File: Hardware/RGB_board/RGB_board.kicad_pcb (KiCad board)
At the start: 2 copper layers, 65 x 56.5 mm, 35 parts, among them J1 PI_HAT_3, J10 Conn_01x02, J2 Screw_Terminal_01x02, J3 Screw_Terminal_01x04, J4 Screw_Terminal_01x02, J5 Conn_01x02, J6 Conn_01x02, J7 Conn_01x02, J8 Conn_01x04, J9 Conn_01x04, Q1 Si1308EDL, Q2 Si1308EDL, Q3 Si1308EDL, Q4 Si1308EDL, SW1 SW_SPDT, SW2 SW_Push_SPST, U1 VO615A-2X009T, U2 VO615A-2X009T, U3 VO615A-2X009T

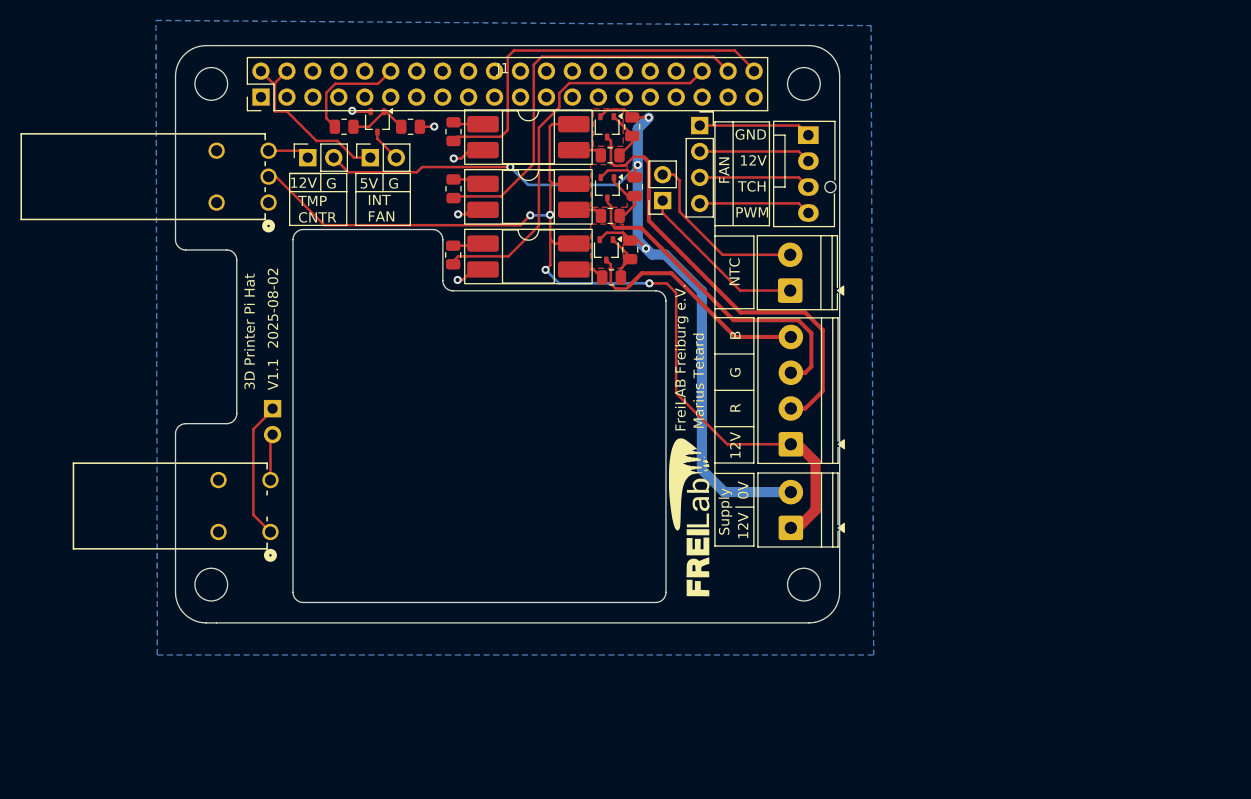
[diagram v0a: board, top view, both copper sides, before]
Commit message: große fortschritte, mockup bereit
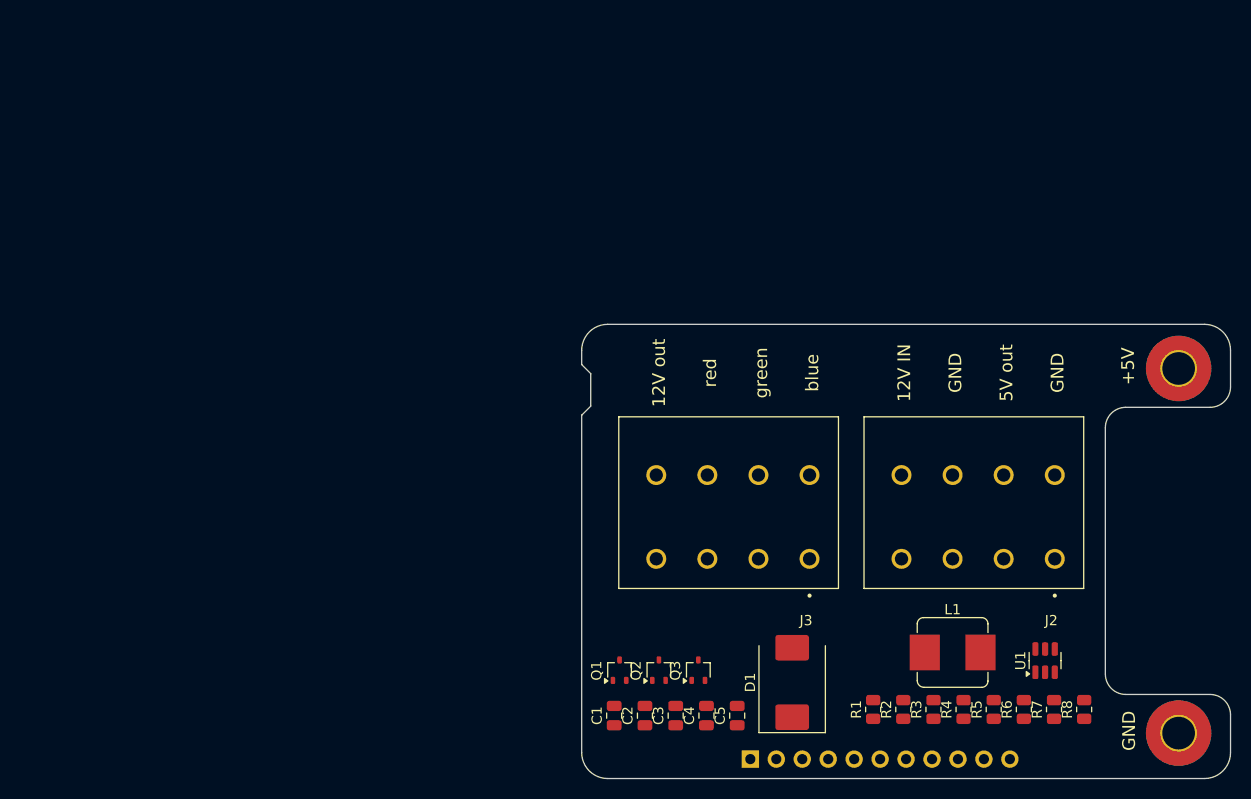
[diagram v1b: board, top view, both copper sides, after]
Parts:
- removed G***: LOGO, aa_MyParts:Freilab_Logo_4mm
- removed H3, H4: MountingHole, MountingHole:MountingHole_3.2mm_M3_DIN965
- removed J10, J5, J6, J7: Conn_01x02, Connector_PinSocket_2.54mm:PinSocket_1x02_P2.54mm_Vertical
- removed J4: Screw_Terminal_01x02, TerminalBlock_Phoenix:TerminalBlock_Phoenix_PT-1,5-2-3.5-H_1x02_P3.50mm_Horizontal
- removed J8: Conn_01x04, Connector_PinSocket_2.54mm:PinSocket_1x04_P2.54mm_Vertical
- removed J9: Conn_01x04, Connector:FanPinHeader_1x04_P2.54mm_Vertical
- removed Q4: Si1308EDL, Package_TO_SOT_SMD:SOT-323_SC-70
- removed R10, R11, R9: 1k5, Resistor_SMD:R_0805_2012Metric
- removed SW1: SW_SPDT, aa_MyParts:SW_200MSP1T1B2M6QE_EWI
- removed SW2: SW_Push_SPST, aa_MyParts:SW_800AWSP9M6QE
- removed U2, U3: VO615A-2X009T, Package_DIP:DIP-4_W8.89mm_SMDSocket_LongPads
- added C1: 10uF, Capacitor_SMD:C_0805_2012Metric, F.Cu at (119.9, 121.1)
- added C2: 10uF, Capacitor_SMD:C_0805_2012Metric, F.Cu at (122.9, 121.1)
- added C3: 100nF, Capacitor_SMD:C_0805_2012Metric, F.Cu at (126.0, 121.1)
- added C4: 22uF, Capacitor_SMD:C_0805_2012Metric, F.Cu at (129.0, 121.1)
- added C5: 22uF, Capacitor_SMD:C_0805_2012Metric, F.Cu at (132.0, 121.1)
- added D1: CDBC540-G, Diode_SMD:D_SMC, F.Cu at (137.4, 117.8)
- added L1: 3.3uH, 6A, Inductor_SMD:L_Bourns_SRP7028A_7.3x6.6mm, F.Cu at (153.1, 114.9)
- added U$25: , S3_MATRIXPORTAL_TOP, F.Cu at (116.8, 127.2)
- added U$26: , S3_MATRIXPORTAL_BOT, B.Cu at (180.3, 127.2)
- H1: value MountingHole -> +5V_Screw; footprint MountingHole:MountingHole_3.2mm_M3_DIN965 -> MountingHole:MountingHole_3.2mm_M3_Pad_TopBottom
- H2: value MountingHole -> GND_Screw; footprint MountingHole:MountingHole_3.2mm_M3_DIN965 -> MountingHole:MountingHole_3.2mm_M3_Pad_TopBottom
- J1: value PI_HAT_3 -> Conn_01x11; footprint aa_MyParts:J_FH20x2_2.54 -> aa_MyParts:J_FM11x2_2.5476341-311LF; moved to B.Cu
- J2: value Screw_Terminal_01x02 -> Conn_01x04; footprint TerminalBlock_Phoenix:TerminalBlock_Phoenix_PT-1,5-2-3.5-H_1x02_P3.50mm_Horizontal -> aa_MyParts:T_4_PhoenixContact_LPT_5_4-H-1x04_Horizontal
- J3: value Screw_Terminal_01x04 -> Conn_01x04; footprint TerminalBlock_Phoenix:TerminalBlock_Phoenix_PT-1,5-4-3.5-H_1x04_P3.50mm_Horizontal -> aa_MyParts:T_4_PhoenixContact_LPT_5_4-H-1x04_Horizontal
- R1, R3, R5: value 15k -> 100R
- R7: value 1k5 -> 56k2
- R8: value 680k -> 10k
- U1: value VO615A-2X009T -> TPS563200; footprint Package_DIP:DIP-4_W8.89mm_SMDSocket_LongPads -> Package_TO_SOT_SMD:SOT-23-6
- moved H1 114.0 mm to (175.2, 122.8)
- moved R7 89.9 mm to (163.0, 120.5), turned to 90 degrees
- moved R8 87.2 mm to (165.9, 120.5), turned to 90 degrees
- moved J1 81.1 mm to (132.5, 126.6), turned to -90 degrees
- moved U1 72.0 mm to (162.1, 115.7), turned to 90 degrees
- moved R2 62.9 mm to (148.2, 120.5), turned to 90 degrees
- moved R4 60.4 mm to (154.1, 120.5), turned to 90 degrees
- moved R1 60.0 mm to (145.3, 120.5), turned to 90 degrees
- moved R6 59.2 mm to (160.0, 120.5), turned to 90 degrees
- moved R3 57.7 mm to (151.2, 120.5), turned to 90 degrees
- moved R5 56.5 mm to (157.1, 120.5), turned to 90 degrees
- moved Q1 53.2 mm to (120.5, 116.6), turned to 90 degrees
- moved Q2 47.5 mm to (124.3, 116.6), turned to 90 degrees
- moved H2 46.0 mm to (175.2, 87.1)
- moved Q3 42.1 mm to (128.2, 116.6), turned to 90 degrees
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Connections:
- J1 pad 1: Net-(J1-3V3-Pad1) -> /RESET
- J1 pad 10: unconnected-(J1-GPIO15/RXD-Pad10) -> /3V
- J1 pad 11: unconnected-(J1-GPIO17-Pad11) -> GND
- J1 pad 2: +5V -> /BOOT
- J1 pad 3: unconnected-(J1-SDA/GPIO2-Pad3) -> /DEBUG
- J1 pad 4: +5V -> /TXO
- J1 pad 5: unconnected-(J1-SCL/GPIO3-Pad5) -> /RXI
- J1 pad 6: GND -> /LED_control_red
- J1 pad 7: unconnected-(J1-GCLK0/GPIO4-Pad7) -> /LED_control_green
- J1 pad 8: unconnected-(J1-GPIO14/TXD-Pad8) -> /LED_control_blue
- J1 pad 9: GND -> /A4
- J2 pad 1: +12V_iso -> GND
- J2 pad 2: GND_ISO -> +5V
- J3 pad 1: +12V_iso -> /LED_blue_-
- J3 pad 2: /LED_red_- -> /LED_green_-
- J3 pad 3: /LED_green_- -> /LED_red_-
- J3 pad 4: /LED_blue_- -> +12V
- Q1 pad 2: GND_ISO -> GND
- Q2 pad 2: GND_ISO -> GND
- Q3 pad 2: GND_ISO -> GND
- R1 pad 1: /LED_opt_red -> /LED_control_red
- R2 pad 1: GND_ISO -> GND
- R3 pad 1: /LED_opt_green -> /LED_control_green
- R4 pad 1: GND_ISO -> GND
- R5 pad 1: /LED_opt_blue -> /LED_control_blue
- R6 pad 1: GND_ISO -> GND
- R7 pad 1: /FAN_control -> Net-(U1-VFB)
- R7 pad 2: Net-(Q4-G) -> +5V
- R8 pad 2: Net-(Q4-G) -> Net-(U1-VFB)
- U1 pad 1: Net-(R9-Pad2) -> GND
- U1 pad 2: GND -> Net-(U1-SW)
- U1 pad 3: /LED_opt_red -> +12V
- U1 pad 4: +12V_iso -> Net-(U1-VFB)
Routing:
- net +12V_iso: track 99.3 -> 0.00 mm, vias 4 -> 0
- net GND_ISO: track 96.5 -> 0.00 mm, vias 4 -> 0
- net /LED_red_-: track 44.1 -> 0.00 mm
- net /LED_control_green: track 38.9 -> 0.00 mm
- net /LED_control_blue: track 38.8 -> 0.00 mm
- net /LED_control_red: track 38.2 -> 0.00 mm
- net /LED_green_-: track 31.8 -> 0.00 mm
- net /LED_blue_-: track 23.3 -> 0.00 mm
- net +5V: track 17.5 -> 0.00 mm
- net Net-(J4-Pin_2): track 17.5 -> 0.00 mm
- net Net-(J4-Pin_1): track 16.8 -> 0.00 mm
- net Net-(J10-Pin_1): track 13.5 -> 0.00 mm
- net GND: track 12.0 -> 0.00 mm, vias 5 -> 0
- net Net-(J8-Pin_4): track 11.0 -> 0.00 mm
- net Net-(J8-Pin_3): track 11.0 -> 0.00 mm
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- removed copper zone on B.Cu, net GND
- removed copper zone on F.Cu, net GND_ISO
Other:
- board size 65 x 56.5 mm -> 63.5 x 44.5 mm
- rule pad_to_mask_clearance: 0.051 -> 0
- board text added: "+5V"
- board text added: "12V IN"
- board text added: "12V out"
- board text added: "5V out"
- board text added: "blue"
- board text added: "green"
- board text added: "red"
- board text removed: "${COMMENT1}"
- board text removed: "${COMPANY}"
- board text removed: "${ISSUE_DATE}"
- board text removed: "${REVISION}"
- board text removed: "${TITLE}"
- board text removed: "0V"
- board text removed: "12V"
- board text removed: "5V"
- board text removed: "B"
- board text removed: "FAN"
- board text removed: "G"
- board text removed: "INT FAN"
- board text removed: "NTC"
- board text removed: "PWM"
- board text removed: "R"
- board text removed: "Supply"
- board text removed: "TCH"
- board text removed: "TMP CNTR"
